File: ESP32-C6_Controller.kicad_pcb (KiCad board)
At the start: 4 copper layers, 15 x 25 mm, 54 parts, among them J1 USB4105-GF-A, J2 Conn_01x12, J3 Conn_01x12, SW1 SW_Push, SW2 SW_Push, U1 ESP32-C6, U2 W25Q16JVSSIQ, U3 AZ1117IH-3.3TRG1, U4 ESD122DMYR

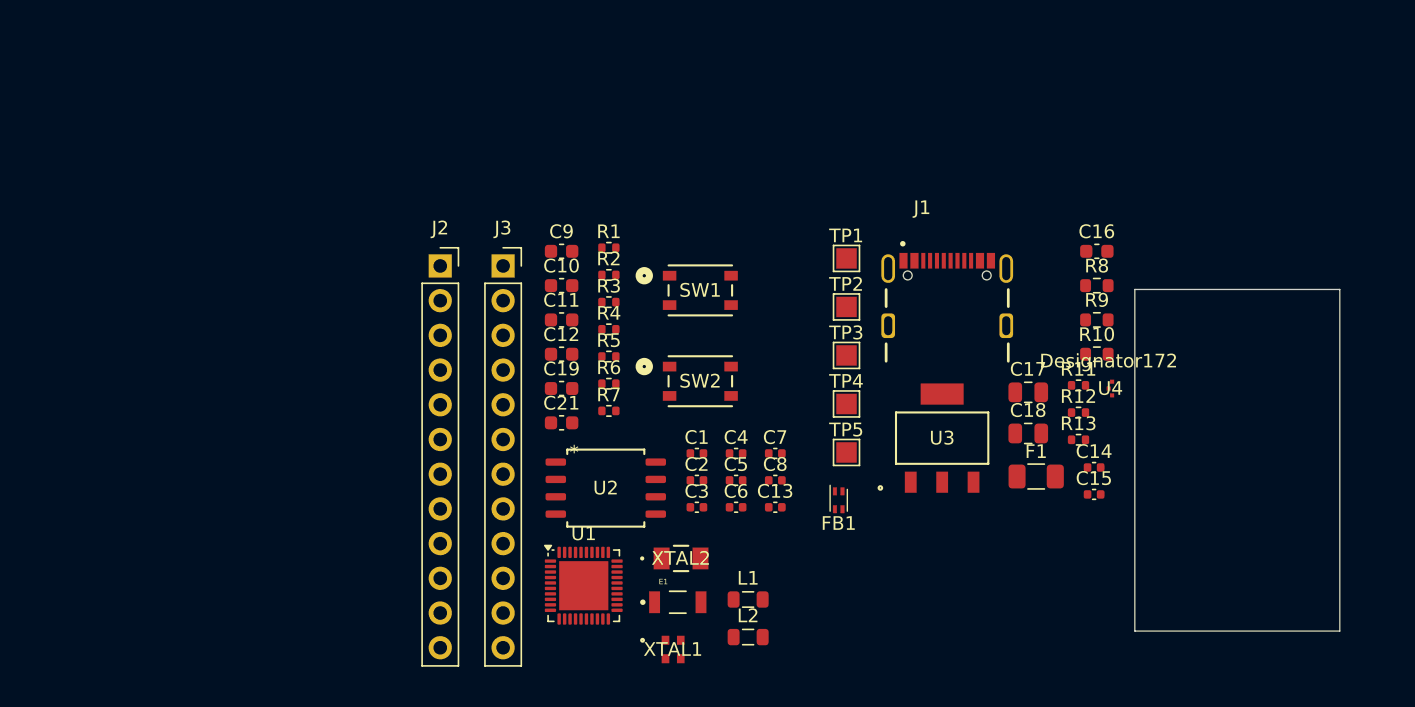
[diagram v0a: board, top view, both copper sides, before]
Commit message: Layout update positions
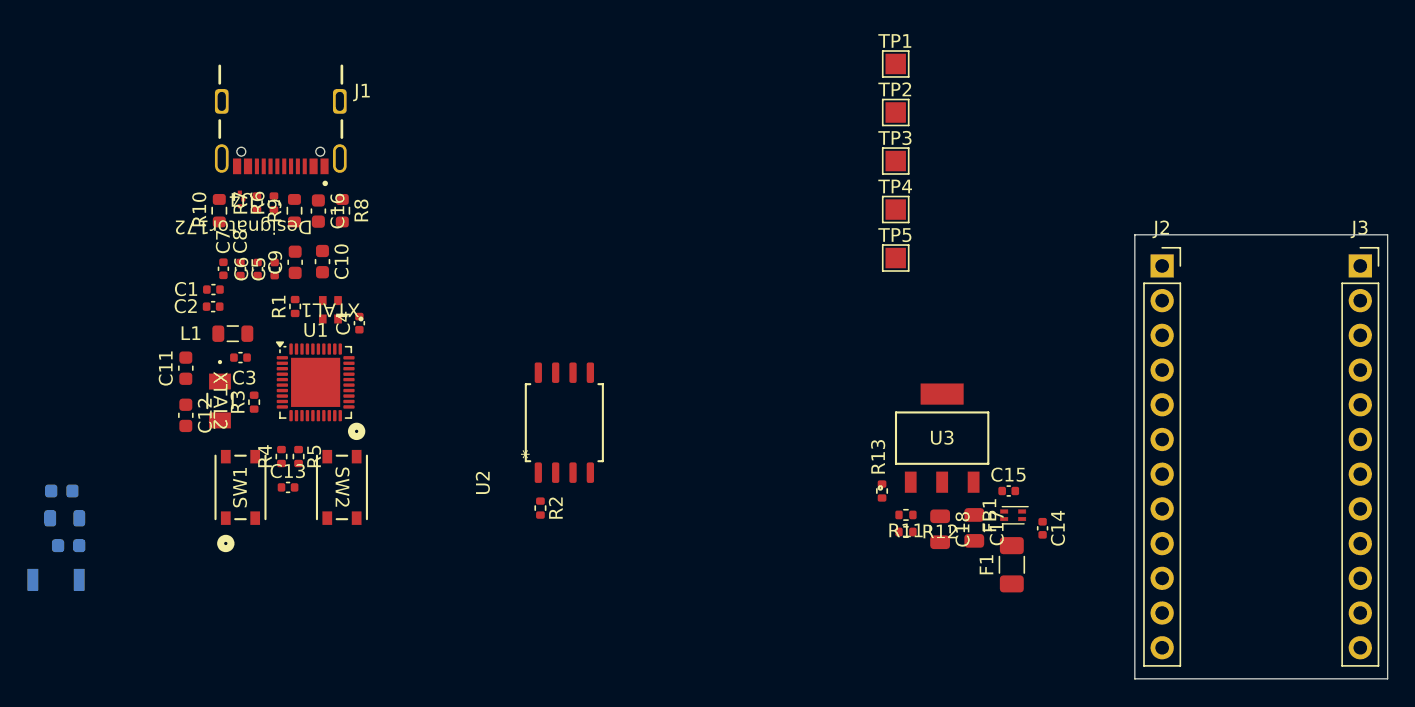
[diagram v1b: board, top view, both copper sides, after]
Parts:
- C19, C21, E1, L2: moved to B.Cu
- moved U4 65.1 mm to (74.6, 93.4), turned to 180 degrees
- moved R10 65.1 mm to (73.0, 94.2), turned to 90 degrees
- moved J3 62.7 mm to (156.5, 98.3)
- moved R9 59.3 mm to (78.5, 94.2), turned to 90 degrees
- moved C16 57.0 mm to (80.2, 94.3), turned to -90 degrees
- moved R8 55.5 mm to (82.0, 94.2), turned to -90 degrees
- moved J2 52.8 mm to (142.0, 98.3)
- moved J1 51.5 mm to (77.5, 86.2), turned to 180 degrees
- moved L2 50.8 mm to (61.7, 116.8), turned to 180 degrees
- moved E1 45.5 mm to (61.0, 121.2), turned to 180 degrees
- moved C7 42.6 mm to (73.3, 98.5), turned to 90 degrees
- moved L1 42.4 mm to (74.0, 103.2), turned to 180 degrees
- moved C8 42.1 mm to (74.5, 98.5), turned to 90 degrees
- moved C6 39.1 mm to (75.8, 98.5), turned to 90 degrees
- moved C19 37.9 mm to (62.0, 118.8), turned to 180 degrees
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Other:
- board size 15 x 25 mm -> 18.5 x 32.5 mm
